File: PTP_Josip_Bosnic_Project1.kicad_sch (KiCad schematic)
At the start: 0 parts

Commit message: ispunjena sastavnica
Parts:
- added R1, R2: R_Small, symbol Device:R_Small
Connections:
- new net +3V3: R1.1
- new net GND: R2.2
- new net U_izl: R1.2, R2.1
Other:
- company: (none) -> TVZ - Tehničko Veleučilište u Zagrebu
- title: (none) -> BCD brojač

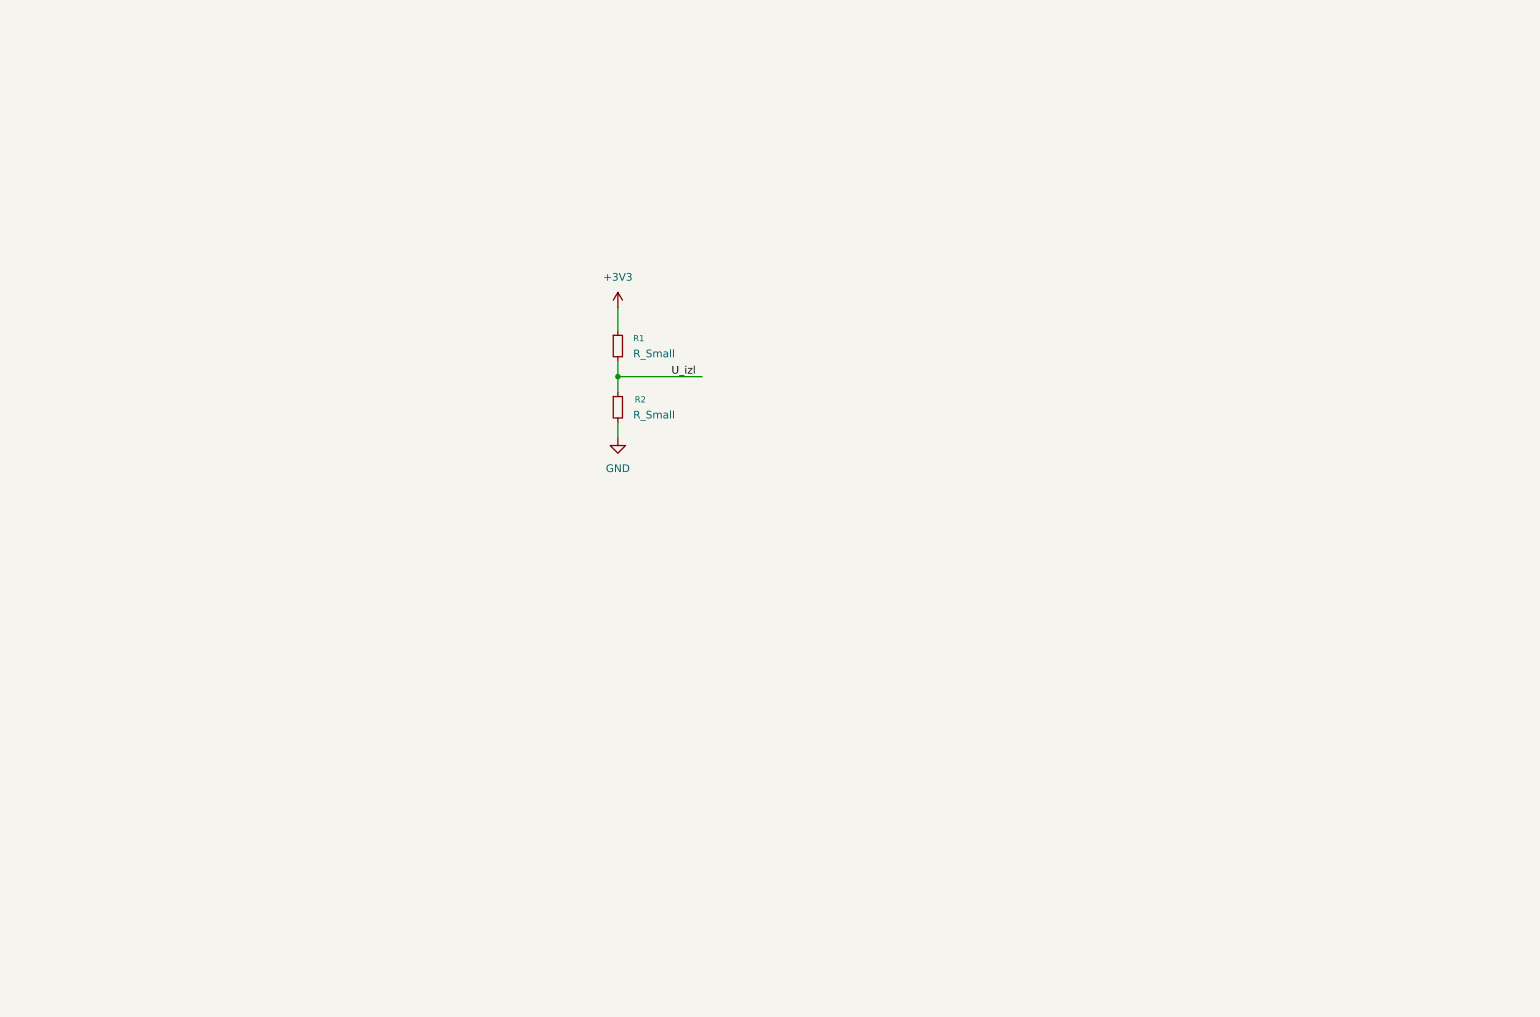
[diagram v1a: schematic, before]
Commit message: Update Sheme
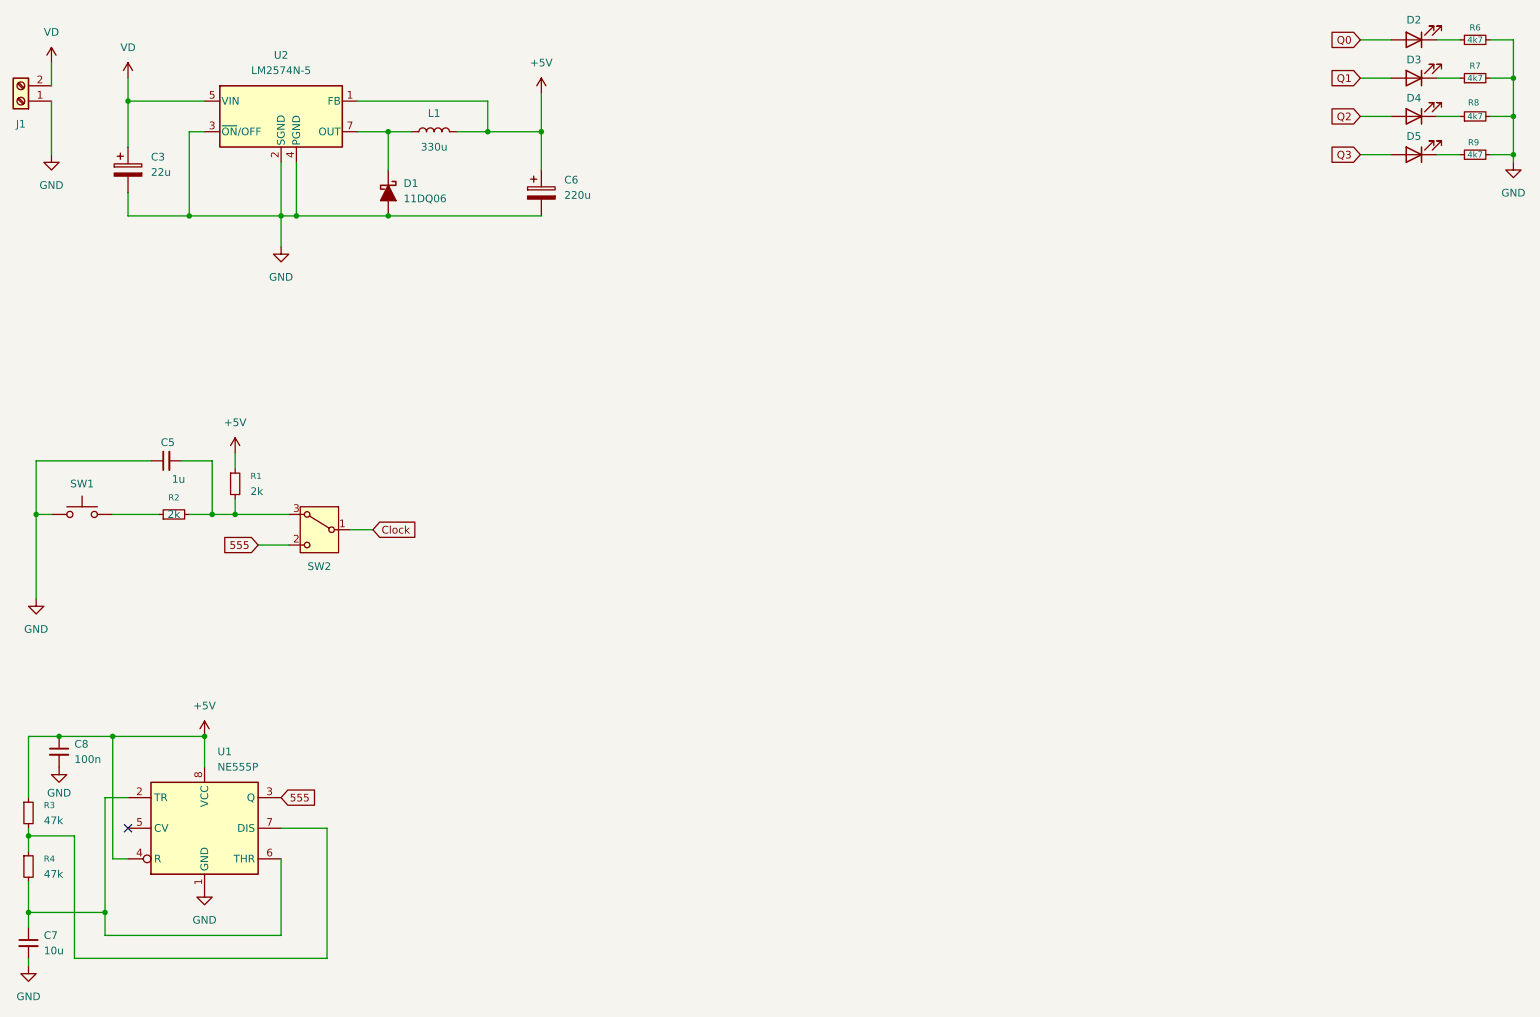
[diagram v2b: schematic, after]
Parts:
- added C3: 22u, symbol Device:C_Polarized
- added C5: 1u, symbol Device:C_Small
- added C6: 220u, symbol Device:C_Polarized
- added C7: 10u, symbol Device:C_Small
- added C8: 100n, symbol Device:C_Small
- added D1: 11DQ06, symbol Device:D_Schottky_Filled
- added D2, D3, D4, D5: LED, symbol Device:LED
- added J1: Screw_Terminal_01x02, symbol Connector:Screw_Terminal_01x02
- added L1: 330u, symbol Device:L
- added R3, R4: 47k, symbol Device:R_Small
- added R6, R7, R8, R9: 4k7, symbol Device:R_Small
- added SW1: SW_Push, symbol Switch:SW_Push
- added SW2: SW_SPDT_312, symbol Switch:SW_SPDT_312
- added U1: NE555P, Package_DIP:DIP-8_W7.62mm, symbol Timer:NE555P
- added U2: LM2574N-5, Package_DIP:DIP-8_W7.62mm, symbol Regulator_Switching:LM2574N-5
- R1, R2: value R_Small -> 2k
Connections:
- net GND: now also C3.2, C5.1, C6.2, C7.2, C8.2, D1.2 (A), J1.1 (Pin_1), R6.2, R7.2, R8.2, R9.2, SW1.1, U1.1 (GND), U2.2 (SGND), U2.3 (~{ON}/OFF), U2.4 (PGND); no longer R2.2
- net +3V3 renamed +5V
- net +5V: now also C6.1, C8.1, L1.2, R3.1, U1.4 (R), U1.8 (VCC), U2.1 (FB)
- net U_izl: no longer names the net of R2.1
- net U_izl: now also SW1.2; no longer R1.2
- new net: D5.1 (K), R9.1
- new net: D2.1 (K), R6.1
- new net: C5.2, R1.2, R2.2, SW2.3 (A)
- new net: C7.1, R4.2, U1.2 (TR), U1.6 (THR)
- new net: R3.2, R4.1, U1.7 (DIS)
- new net: D4.1 (K), R8.1
- new net: D3.1 (K), R7.1
- new net: D1.1 (K), L1.1, U2.7 (OUT)
- new net 555: SW2.2 (C), U1.3 (Q)
- new net Clock: SW2.1 (B)
- new net Q0: D2.2 (A)
- new net Q1: D3.2 (A)
- new net Q2: D4.2 (A)
- new net Q3: D5.2 (A)
- new net VD: C3.1, J1.2 (Pin_2), U2.5 (VIN)
- no-connect marks 0 -> 1
